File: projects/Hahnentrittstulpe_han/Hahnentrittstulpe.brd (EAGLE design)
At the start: 100 x 80 mm, 10 parts, among them IC1 TINY13-20SU

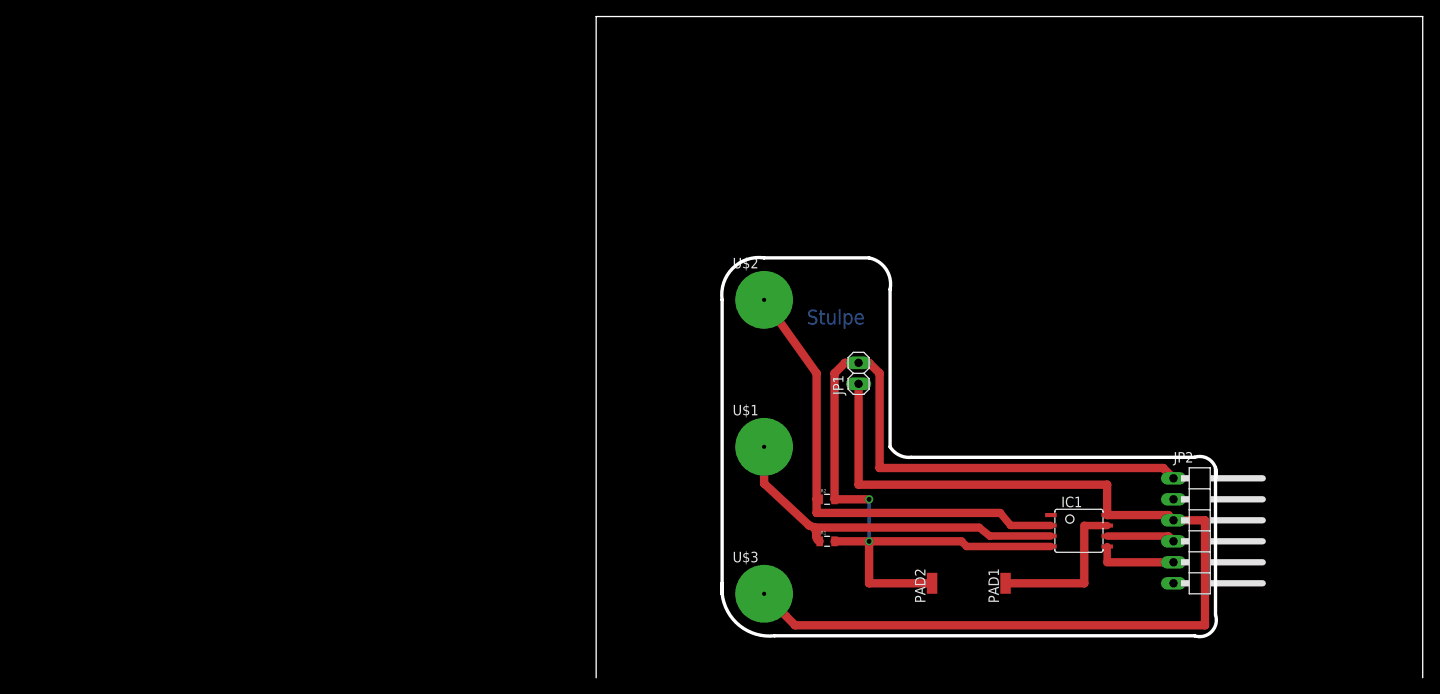
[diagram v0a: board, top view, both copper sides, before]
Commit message: final stulpe
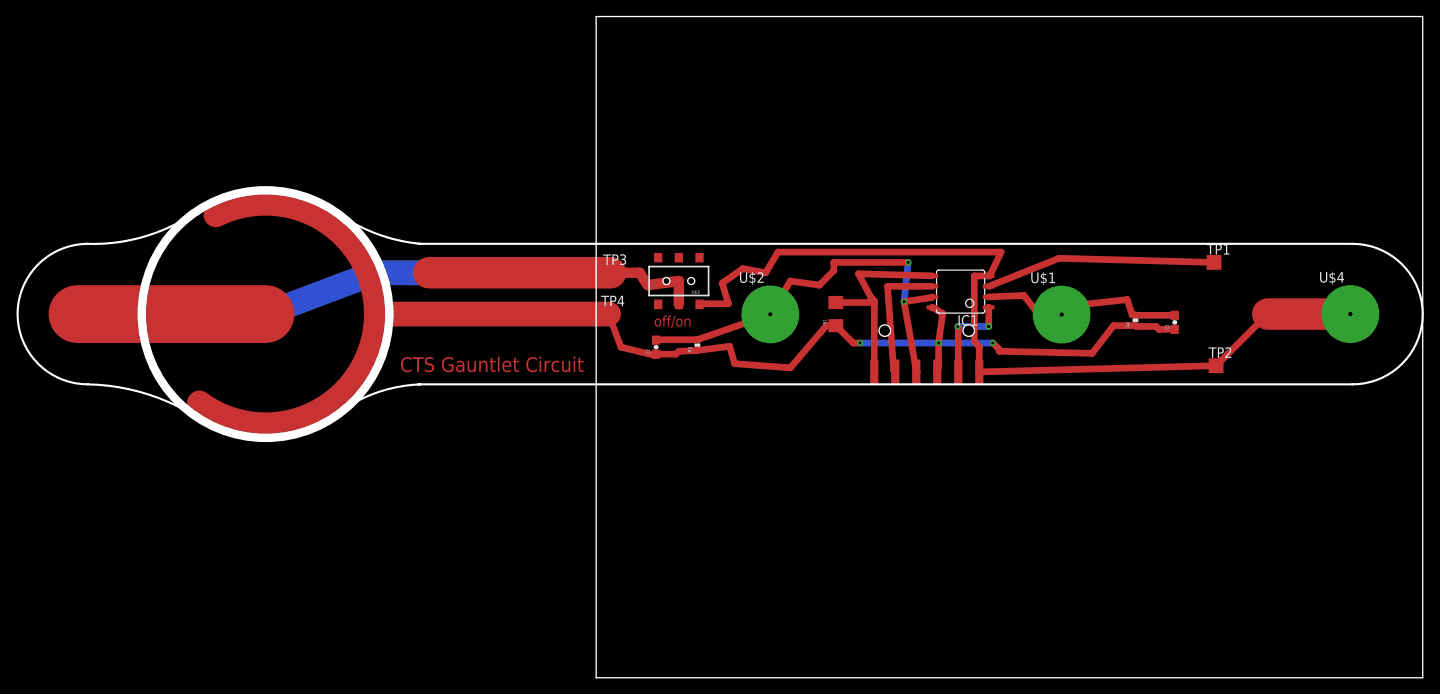
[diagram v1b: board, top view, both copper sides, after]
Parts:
- removed JP2: (no value), pinhead:1X06/90
- removed PAD1, PAD2: (no value), wirepad:SMD1,27-2,54
- removed R2: (no value), SparkFun-Resistors:0805
- added C1, C2: (no value), SparkFun-Capacitors:0603-CAP
- added R3, R4: (no value), SparkFun-Passives:0402-RES
- added TP1, TP2, TP3, TP4: TPTP18SQ, testpad:TP18SQ
- added U$4: SNAP-PAD_7MM_ROUND, hannahsEagleLib:SNAP-PAD_7MM_RD
- JP1: device pinhead:1X02 -> SparkFun-Connectors:1X06-SMD
- R1: device SparkFun-Resistors:0805 -> SparkFun-Resistors:1206
- U$3: value SNAP-PAD_7MM_ROUND -> AYZ0202; device hannahsEagleLib:SNAP-PAD_7MM_RD -> SparkFun-Electromechanical:AYZ0202
- moved U$1 39.4 mm to (56.3, 43.9)
- moved U$3 39.2 mm to (10.0, 48.0), turned to 180 degrees
- moved IC1 32.3 mm to (44.1, 46.7), turned to 90 degrees
- moved R1 27.5 mm to (29.0, 44.0), turned to 90 degrees
- moved JP1 9.74 mm to (40.0, 42.0), turned to 180 degrees
- moved U$2 1.90 mm to (21.1, 44.0)
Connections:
- removed net N$4: IC1.7, PAD1.1
- removed net N$9: IC1.4, JP1.2, JP2.1, PAD2.1, R1.2, R2.2
- new net N$1: IC1.1, JP1.2
- new net N$10: IC1.6, JP1.5
- new net N$11: IC1.5, JP1.6, R1.2
- new net N$21: TP3.TP, U$3.2
- net N$2: now also TP1.TP; no longer R1.1, U$1.P$1
- net N$3: now also C1.2, R4.2, U$1.P$1; no longer R2.1, U$2.P$1
- net N$5: now also C2.2, IC1.7, JP1.4, R3.2, U$2.P$1; no longer IC1.8, JP1.1, JP2.3, U$3.P$1
- net N$6: now also IC1.4, JP1.1, TP2.TP, U$3.1, U$4.P$1; no longer IC1.6, JP2.4
- net N$7: now also C1.1, C2.1, IC1.8, JP1.3, R1.1, R3.1, R4.1, TP4.TP; no longer IC1.5, JP2.5
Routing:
- net N$9: track 117.7 -> 0.00 mm, vias 2 -> 0
- net N$7: track 9.93 -> 115.5 mm, vias 0 -> 2
- net N$6: track 8.29 -> 106.3 mm
- net N$5: track 125.7 -> 52.0 mm, vias 0 -> 2
- net N$15: track 0.00 -> 42.7 mm
- net N$21: track 0.00 -> 33.9 mm
- net N$3: track 57.2 -> 25.5 mm
- net N$11: track 0.00 -> 26.1 mm
- net N$18: track 0.00 -> 22.8 mm
- net N$20: track 0.00 -> 22.8 mm
- net N$4: track 19.3 -> 0.00 mm
- net N$10: track 0.00 -> 15.9 mm
- net N$2: track 43.3 -> 27.9 mm
- net N$1: track 0.00 -> 11.7 mm, vias 0 -> 1
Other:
- board size 100 x 80 mm -> 170 x 80 mm
- board text added: "CTS Gauntlet Circuit"
- board text added: "off/on"
- board text removed: "Stulpe"
